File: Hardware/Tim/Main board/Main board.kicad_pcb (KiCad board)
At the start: 4 copper layers, 113 x 65.5 mm, 186 parts, among them J1 SOICbite, J10 Conn_01x03_Socket, J11 Nichrome, J12 USB_C_Receptacle_USB2.0, J13 Conn_01x02_Socket, J14 Conn_01x02_Pin, J15 Conn_01x04_Socket, J16 Conn_01x02_Pin, J2 USB_C_Receptacle_USB2.0, J3 Conn_01x04_Socket, J4 Conn_01x04_Socket, J5 Conn_01x04_Socket, J6 Conn_01x02_Socket, J7 Conn_01x02_Socket, J8 U.FL, J9 SOICbite, Q1 IRLML0060TRPBF, Q2 IRLML0060TRPBF, U1 RP2040, U10 MAX-M10S, U11 ADP7105ACPZ-5.0-R7, U12 ADP7105ACPZ-3.3-R7, U13 ADP7105ACPZ-5.0-R7, U14 TPS2121RUXR, U15 TPS2121RUXR, U2 W25Q64JVZP, U3 MS5607-02BA, U4 BMI270, U5 ADP7105ACPZ-3.3-R7, U6 DRF1262TL, U7 RP2040, U8 W25Q64JVZP, U9 LT3120JV-PBF, Y1 445I23D12M00000, Y3 445I23D12M00000

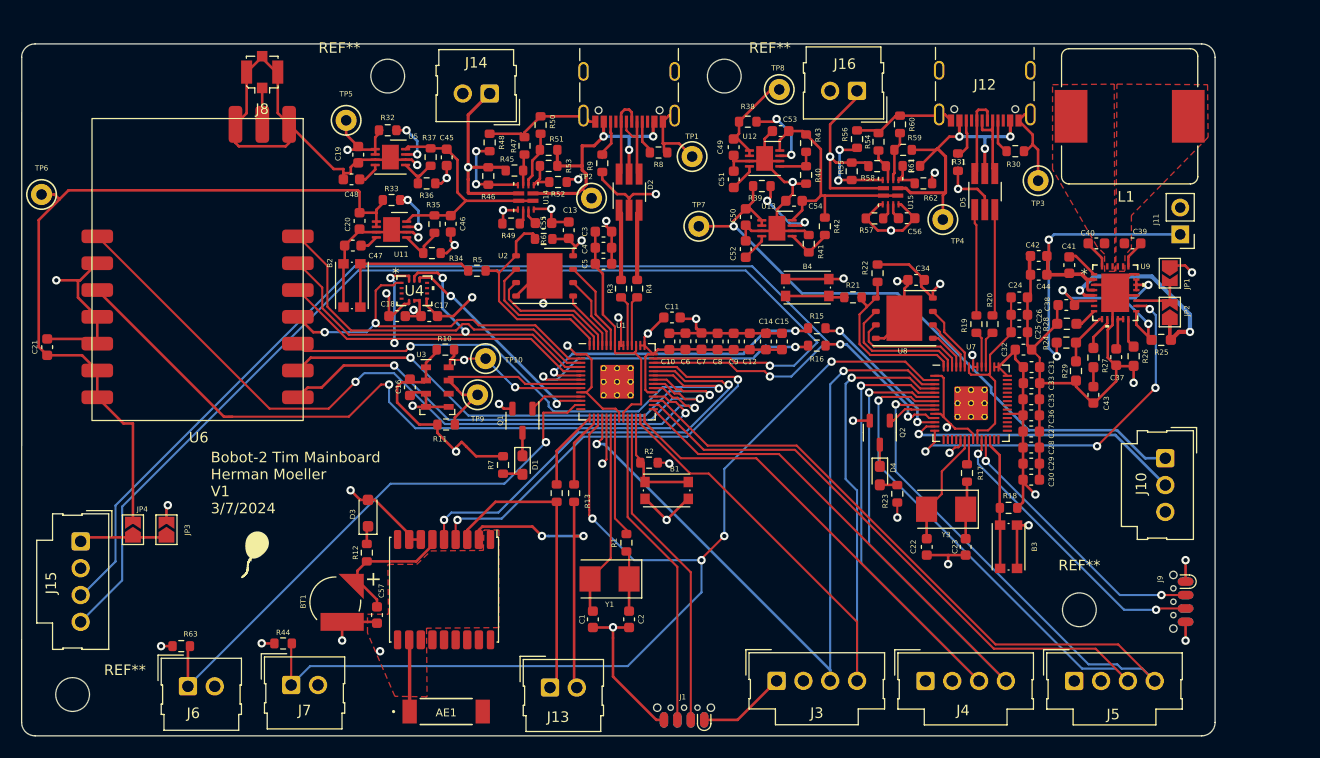
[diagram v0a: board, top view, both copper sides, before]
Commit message: Update changes hopefully good
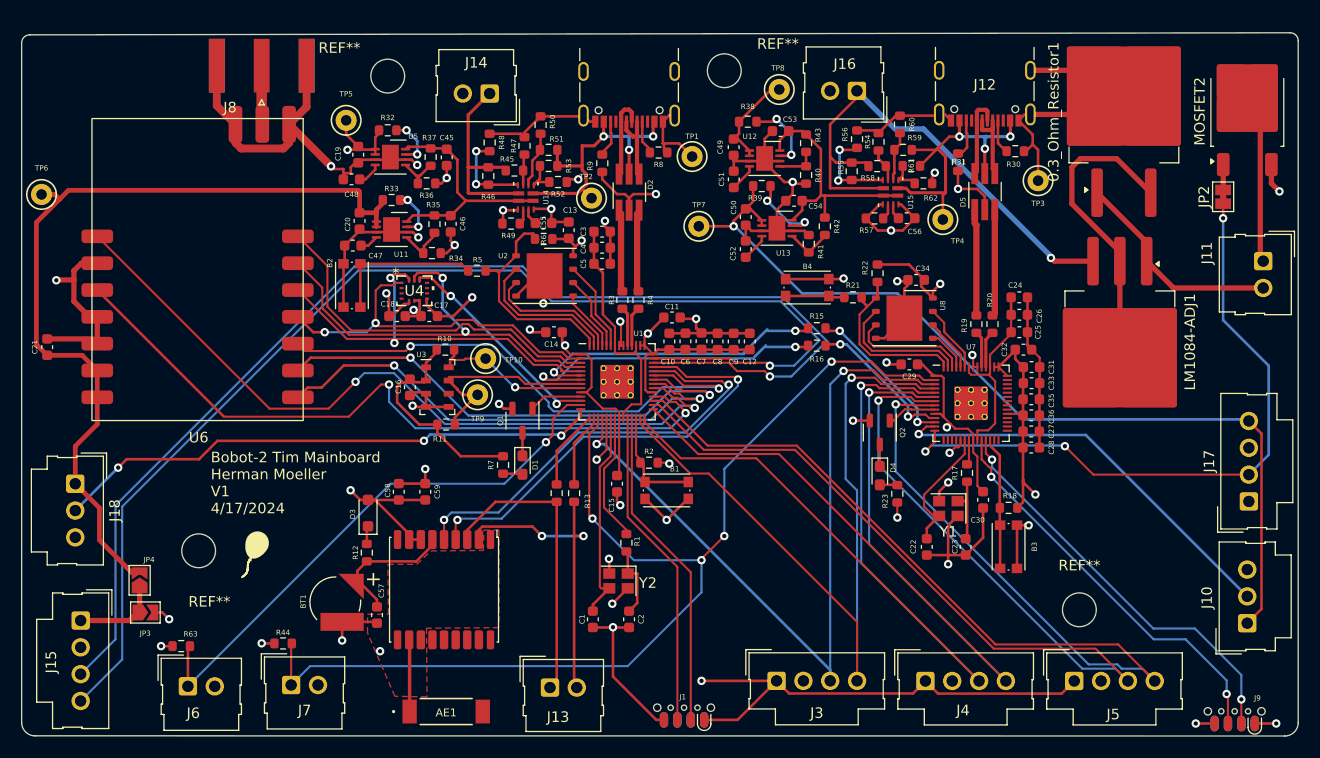
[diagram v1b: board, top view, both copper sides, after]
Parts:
- removed C37: 4.7uF, Capacitor_SMD:C_0603_1608Metric
- removed C38: 10uF, Capacitor_SMD:C_0603_1608Metric
- removed C39, C40: 220nF, Capacitor_SMD:C_0603_1608Metric
- removed C41: 22nF, Capacitor_SMD:C_0603_1608Metric
- removed C42, C44: 22uF, Capacitor_SMD:C_0603_1608Metric
- removed C43: 680p, Capacitor_SMD:C_0603_1608Metric
- removed JP1: SolderJumper_2_Open, Jumper:SolderJumper-2_P1.3mm_Open_TrianglePad1.0x1.5mm
- removed L1: 3.3uH, BPPlib:L_Bourns_SRP1265A
- removed R24: 81.1k, Resistor_SMD:R_0603_1608Metric_Pad0.98x0.95mm_HandSolder
- removed R25: 5m, Resistor_SMD:R_0603_1608Metric_Pad0.98x0.95mm_HandSolder
- removed R26: 75k, Resistor_SMD:R_0603_1608Metric_Pad0.98x0.95mm_HandSolder
- removed R27: 56.2k, Resistor_SMD:R_0603_1608Metric_Pad0.98x0.95mm_HandSolder
- removed R28, R29: 154k, Resistor_SMD:R_0603_1608Metric_Pad0.98x0.95mm_HandSolder
- removed U9: LT3120JV-PBF, BPPlib:LQFN28_Rev0_ADI
- removed Y3: 445I23D12M00000, Crystal:Crystal_SMD_5032-2Pin_5.0x3.2mm
- added 0.3_Ohm_Resistor1: 03, Package_TO_SOT_SMD:TO-263-2, F.Cu at (161.5, 60.3)
- added C58: 100nF, Capacitor_SMD:C_0603_1608Metric, F.Cu at (92.9, 96.3)
- added C59: 1uF, Capacitor_SMD:C_0603_1608Metric, F.Cu at (95.4, 96.3)
- added J17: Conn_01x04_Pin, Connector_Molex:Molex_SL_171971-0004_1x04_P2.54mm_Vertical, F.Cu at (173.4, 97.2)
- added J18: Conn_01x03_Socket, Connector_Molex:Molex_SL_171971-0003_1x03_P2.54mm_Vertical, F.Cu at (62.2, 95.5)
- added LM1084-ADJ1: LM1084-ADJ, Package_TO_SOT_SMD:TO-263-3_TabPin2, F.Cu at (161.2, 82.1)
- added MOSFET2: IRF540N, Package_TO_SOT_SMD:TO-252-2, F.Cu at (173.2, 60.2)
- added Y2: 12MHz, Crystal:Crystal_SMD_2520-4Pin_2.5x2.0mm, F.Cu at (113.7, 104.7)
- C1, C2, C22, C23: value 22pF -> 10pF
- J11: value Nichrome -> Conn_01x02_Pin; footprint Connector_PinHeader_2.54mm:PinHeader_1x02_P2.54mm_Vertical -> Connector_Molex:Molex_SL_171971-0002_1x02_P2.54mm_Vertical
- J8: footprint Connector_Coaxial:U.FL_Molex_MCRF_73412-0110_Vertical -> Connector_Coaxial:SMA_Amphenol_132289_EdgeMount
- JP2: value SolderJumper_2_Open -> SolderJumper_2_Bridged; footprint Jumper:SolderJumper-2_P1.3mm_Open_TrianglePad1.0x1.5mm -> Jumper:SolderJumper-2_P1.3mm_Bridged_Pad1.0x1.5mm
- Y1: value 445I23D12M00000 -> 12MHz; footprint Crystal:Crystal_SMD_5032-2Pin_5.0x3.2mm -> Crystal:Crystal_SMD_2520-4Pin_2.5x2.0mm
- moved Y1 32.8 mm to (144.9, 97.9)
- moved C15 20.6 mm to (113.5, 95.5), turned to -90 degrees
- moved C14 20.1 mm to (107.6, 81.2), turned to 180 degrees
- moved REF** 18.1 mm to (73.9, 101.9)
- moved J10 17.4 mm to (173.2, 108.7), turned to 90 degrees
- moved C29 14.9 mm to (141.2, 84.2), turned to 180 degrees
- moved J9 12.9 mm to (172.0, 119.0), turned to 0 degrees
- moved JP2 12.0 mm to (170.9, 68.3)
- moved J11 8.26 mm to (174.7, 74.4), turned to -90 degrees
- moved JP3 8.09 mm to (68.9, 107.7), turned to 0 degrees
- moved J15 7.49 mm to (62.7, 108.5)
- moved C30 4.94 mm to (148.2, 97.0), turned to -90 degrees
- moved JP4 4.83 mm to (68.3, 104.6)
- moved R3 1.09 mm to (114.0, 78.1)
- moved R4 1.09 mm to (115.6, 78.1)
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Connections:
- C27 pad 1: +3V3 -> +3V3_R
- C28 pad 1: +3V3 -> +3V3_R
- C29 pad 1: +3V3 -> +3V3_R
- C30 pad 1: +3V3 -> +3V3_R
- C31 pad 1: +3V3 -> +3V3_R
- C32 pad 1: +3V3 -> +3V3_R
- C33 pad 1: +3V3 -> +3V3_R
- C34 pad 1: +3V3 -> +3V3_R
- C35 pad 1: +3V3 -> +3V3_R
- C36 pad 1: +3V3 -> +3V3_R
- C49 pad 1: +3V3 -> +3V3_R
- C50 pad 1: +5V -> +5V_R
- J10 pad 1: +5V -> +5V_R
- J11 pad 2: GND -> Net-(J11-Pin_2)
- J16 pad 1: Net-(J16-Pin_1) -> +BATT
- J9 pad 1: +3V3 -> +3V3_R
- JP2 pad 1: +BATT -> /CUT
- R18 pad 1: +3V3 -> +3V3_R
- R22 pad 1: +3V3 -> +3V3_R
- R23 pad 1: +3V3 -> +3V3_R
- R38 pad 1: +3V3 -> +3V3_R
- R39 pad 1: +5V -> +5V_R
- R55 pad 2: Net-(J16-Pin_1) -> +BATT
- R58 pad 2: Net-(J16-Pin_1) -> +BATT
- TP7 pad 1: +5V -> +5V_R
- TP8 pad 1: +3V3 -> +3V3_R
- U12 pad 1: +3V3 -> +3V3_R
- U12 pad 2: +3V3 -> +3V3_R
- U13 pad 1: +5V -> +5V_R
- U13 pad 2: +5V -> +5V_R
- U15 pad 7: Net-(J16-Pin_1) -> +BATT
- U7 pad 1: +3V3 -> +3V3_R
- U7 pad 10: +3V3 -> +3V3_R
- U7 pad 22: +3V3 -> +3V3_R
- U7 pad 33: +3V3 -> +3V3_R
- U7 pad 42: +3V3 -> +3V3_R
- U7 pad 43: +3V3 -> +3V3_R
- U7 pad 44: +3V3 -> +3V3_R
- U7 pad 48: +3V3 -> +3V3_R
- U7 pad 49: +3V3 -> +3V3_R
- U8 pad 8: +3V3 -> +3V3_R
- Y1 pad 1: Net-(C2-Pad2) -> Net-(C23-Pad2)
- Y1 pad 2: Net-(U1-XIN) -> GND
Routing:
- net +5V_R: track 0.00 -> 87.0 mm, vias 0 -> 1
- net +3V3_R: track 0.00 -> 63.4 mm, vias 0 -> 6
- net +5V: track 135.3 -> 81.5 mm, vias 1 -> 0
- net /PWM_MC: track 0.00 -> 52.3 mm, vias 0 -> 3
- net +BATT: track 19.7 -> 49.4 mm, vias 2 -> 1
- net Net-(LM1084-ADJ1-VO): track 0.00 -> 29.1 mm
- net /CUT: track 35.8 -> 62.6 mm, vias 4 -> 3
- net Net-(U9-ISN): track 23.2 -> 0.00 mm, vias 3 -> 0
- net Net-(J11-Pin_1): track 34.8 -> 14.0 mm, vias 2 -> 0
- net Net-(J11-Pin_2): track 0.00 -> 20.5 mm
- net Net-(J16-Pin_1): track 20.2 -> 0.00 mm, vias 1 -> 0
- net /SWD_R: track 26.2 -> 39.2 mm
- net +3V3: track 162.5 -> 149.8 mm, vias 20 -> 13
- net /PWM_EMRG_REL: track 27.3 -> 39.4 mm
- net /SWCLK_R: track 27.9 -> 38.3 mm
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- added copper zone on In2.Cu, net +3V3_R
- removed copper zone on F.Cu, net Net-(C39-Pad2)
- removed copper zone on F.Cu, net Net-(C40-Pad2)
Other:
- board size 113 x 65.5 mm -> 120.9 x 66.6 mm
- board text added: "Bobot-2 Tim Mainboard Herman Moeller V1 4/17/2024"
- board text removed: "Bobot-2 Tim Mainboard Herman Moeller V1 3/7/2024"
